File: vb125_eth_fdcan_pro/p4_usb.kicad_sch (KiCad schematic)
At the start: 19 parts, among them J3 USB_C_Receptacle_USB2.0, Q1 BSS138, Q2 BSS138, U3 USB3315, X1 24MHz

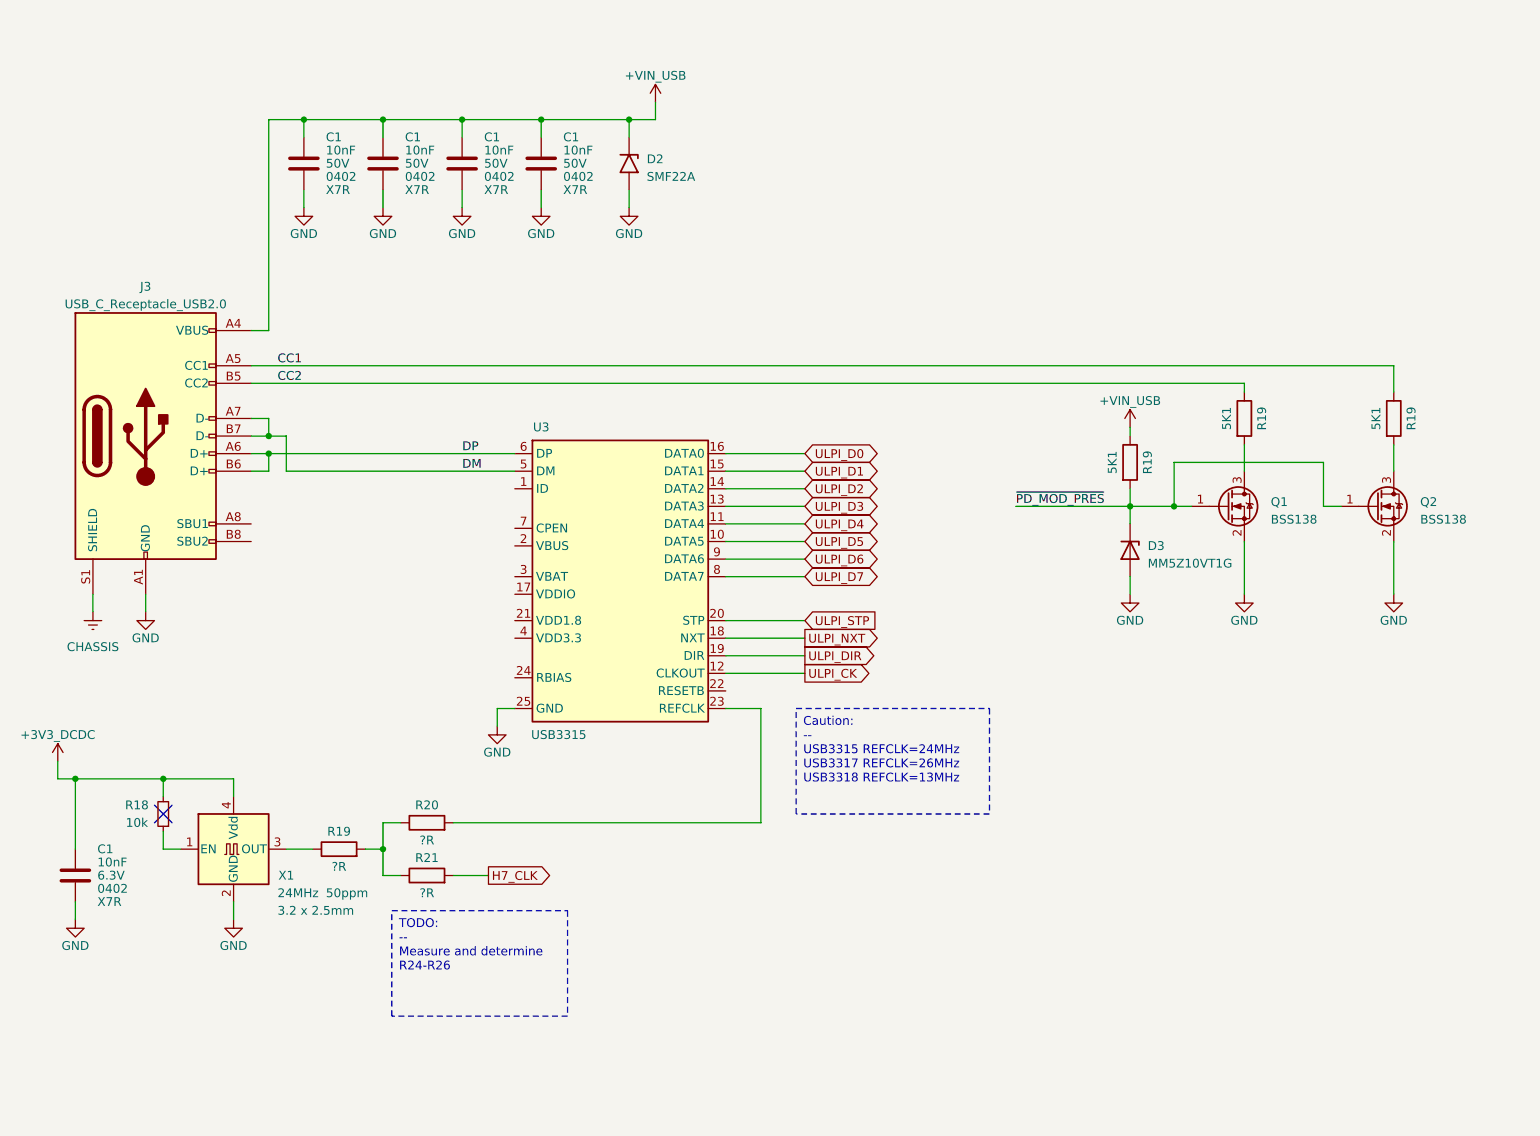
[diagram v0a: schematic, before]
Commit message: Finish schematics.
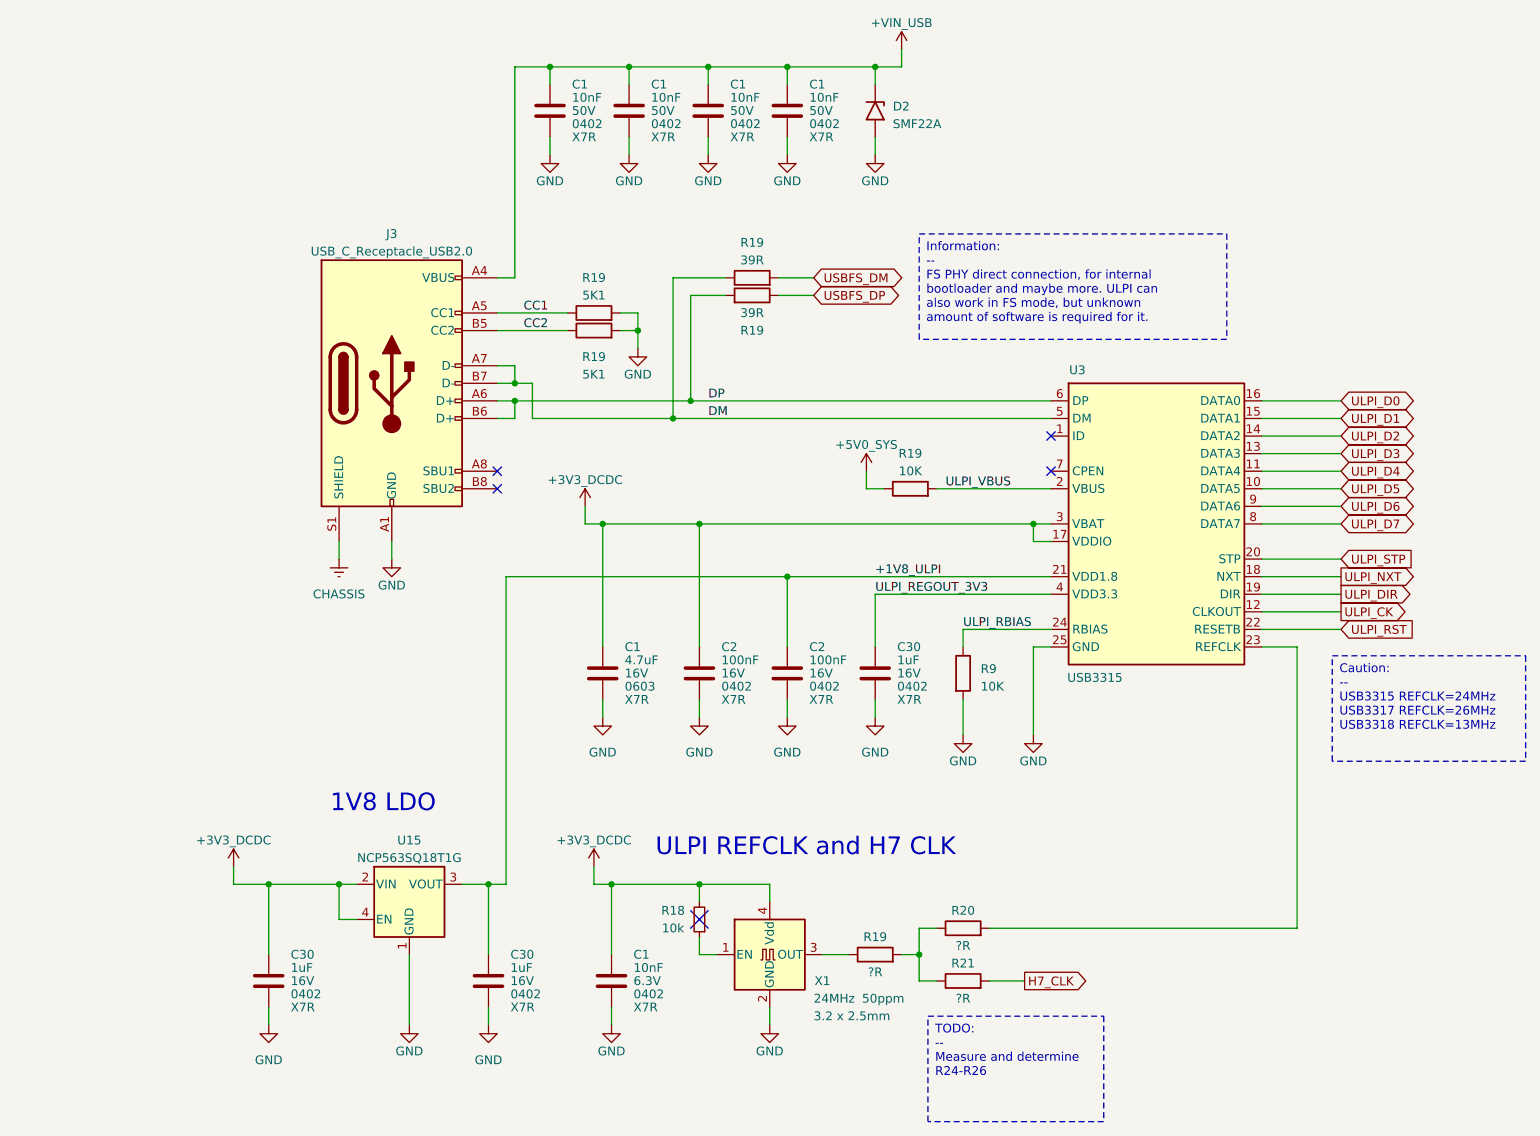
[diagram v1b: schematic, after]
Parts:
- removed D3: MM5Z10VT1G, Diode_SMD:D_SOD-523, symbol Diode:MM5Zxx
- removed Q1, Q2: BSS138, Package_TO_SOT_SMD:SOT-23, symbol Transistor_FET:BSS138
- removed R19: 5K1, Resistor_SMD:R_0402_1005Metric, symbol Device:R
- added C1: 4.7uF, Capacitor_SMD:C_0603_1608Metric, symbol Device:C
- added C2 (x2): 100nF, Capacitor_SMD:C_0402_1005Metric, symbol Device:C
- added C30 (x3): 1uF, Capacitor_SMD:C_0402_1005Metric, symbol Device:C
- added R19 (x2): 39R, Resistor_SMD:R_0402_1005Metric, symbol Device:R
- added R19, R9: 10K, Resistor_SMD:R_0402_1005Metric, symbol Device:R
- added U15: NCP563SQ18T1G, Package_TO_SOT_SMD:SC-82AB, symbol Regulator_Linear:NCP662SQ18
- C1: footprint (none) -> Capacitor_SMD:C_0402_1005Metric
- R18: footprint (none) -> Resistor_SMD:R_0402_1005Metric
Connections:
- net +3V3_DCDC: now also U3.17 (VDDIO), U3.3 (VBAT), C1.1, C2.1, C30.1, U15.2 (VIN), U15.4 (EN)
- net DM: now also R19.1
- net DP: now also R19.2
- net GND: now also R19.2, R19.2, C1.2, C2.2, C2.2, C30.2, C30.2, C30.2, R9.2, U15.1 (GND)
- net ULPI_VBUS: now reaches U3.2 (VBUS)
- net ULPI_VBUS: now also R19.2
- net +1V8_ULPI: now reaches U3.21 (VDD1.8)
- net +1V8_ULPI: now also C2.1, C30.1, U15.3 (VOUT)
- net ULPI_RST: now reaches U3.22 (RESETB)
- net ULPI_RBIAS: now reaches U3.24 (RBIAS)
- net ULPI_RBIAS: now also R9.1
- net ULPI_REGOUT_3V3: now reaches U3.4 (VDD3.3)
- net ULPI_REGOUT_3V3: now also C30.1
- new net +5V0_SYS: R19.1
- new net USBFS_DM: R19.2
- new net USBFS_DP: R19.1
- no-connect marks 0 -> 4
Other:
- note added: "1V8 LDO"
- note added: "ULPI REFCLK and H7 CLK"
- moved on the sheet: C1, D2, J3, R18, R19, R20, R21, U3, X1
